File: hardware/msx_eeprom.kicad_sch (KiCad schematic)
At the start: 8 parts, among them J1 Conn_02x07_Odd_Even, P1 MSX_CONNECTOR, U1 AT28C256-15PU

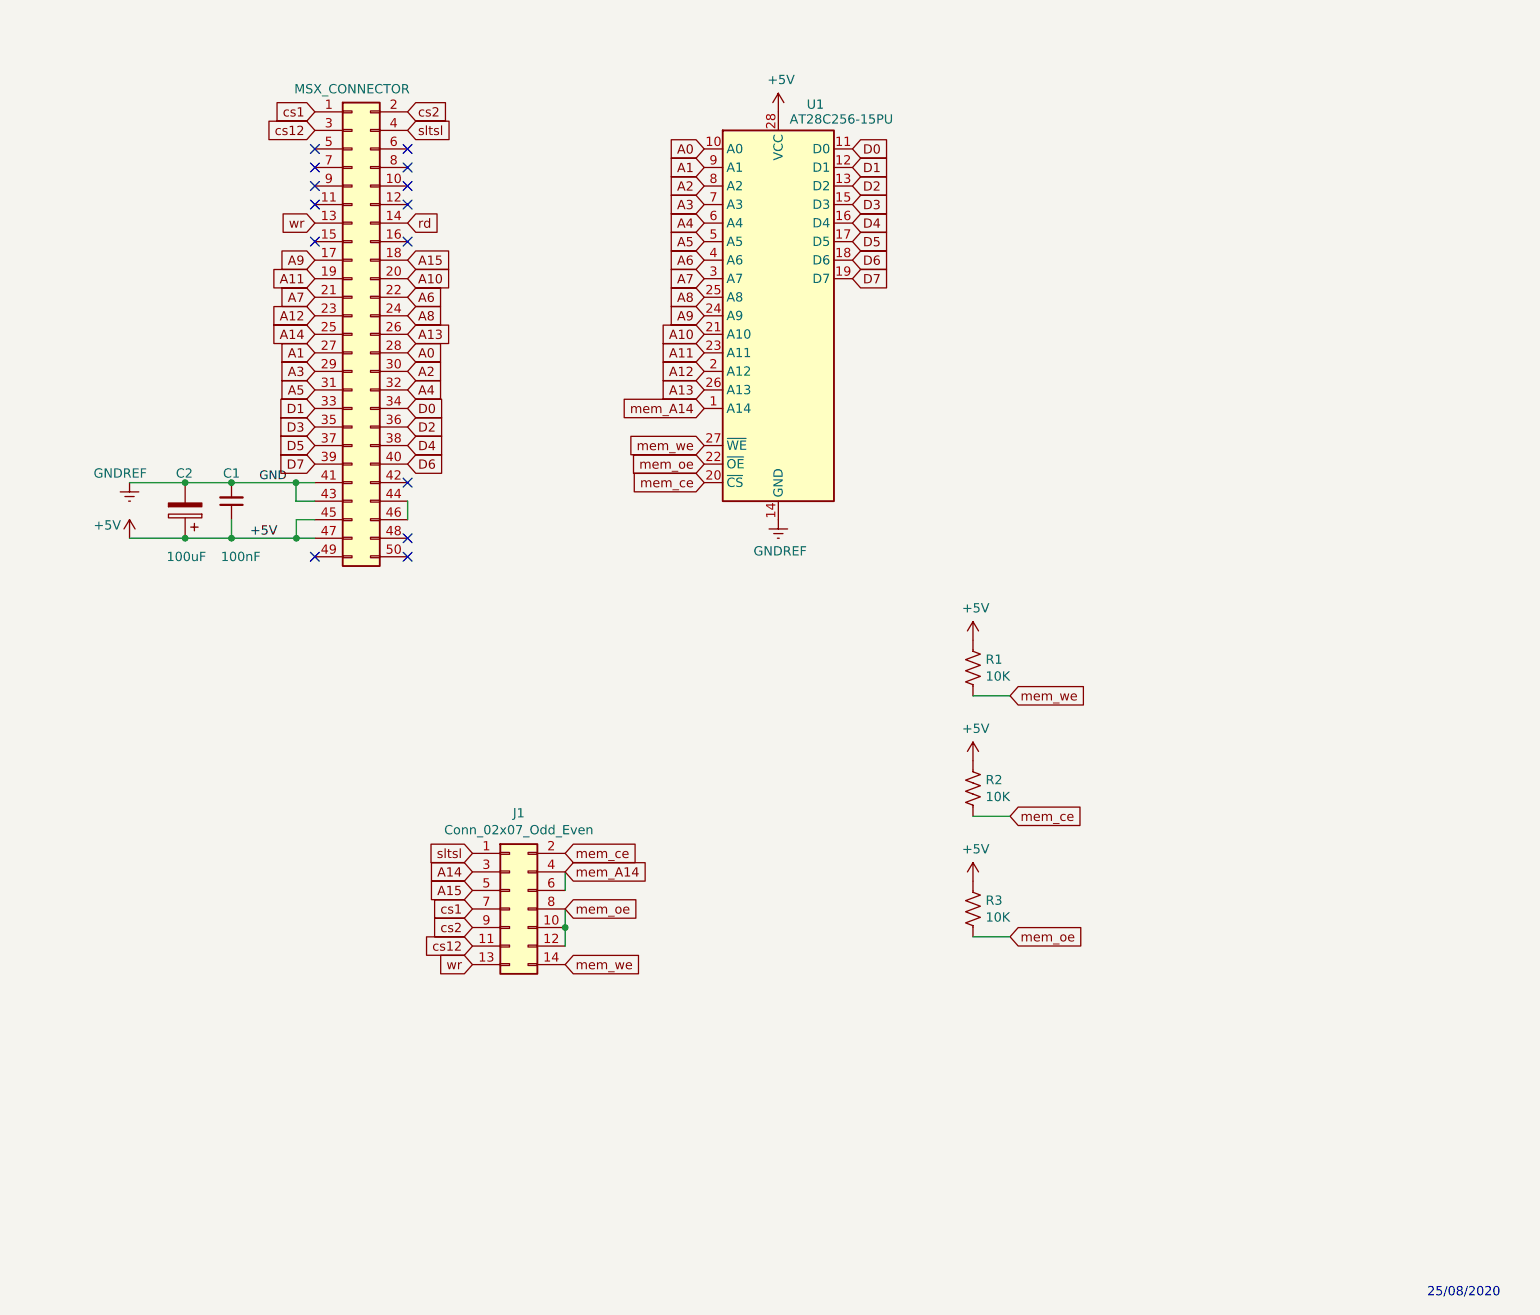
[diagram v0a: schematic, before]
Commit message: Rev 7
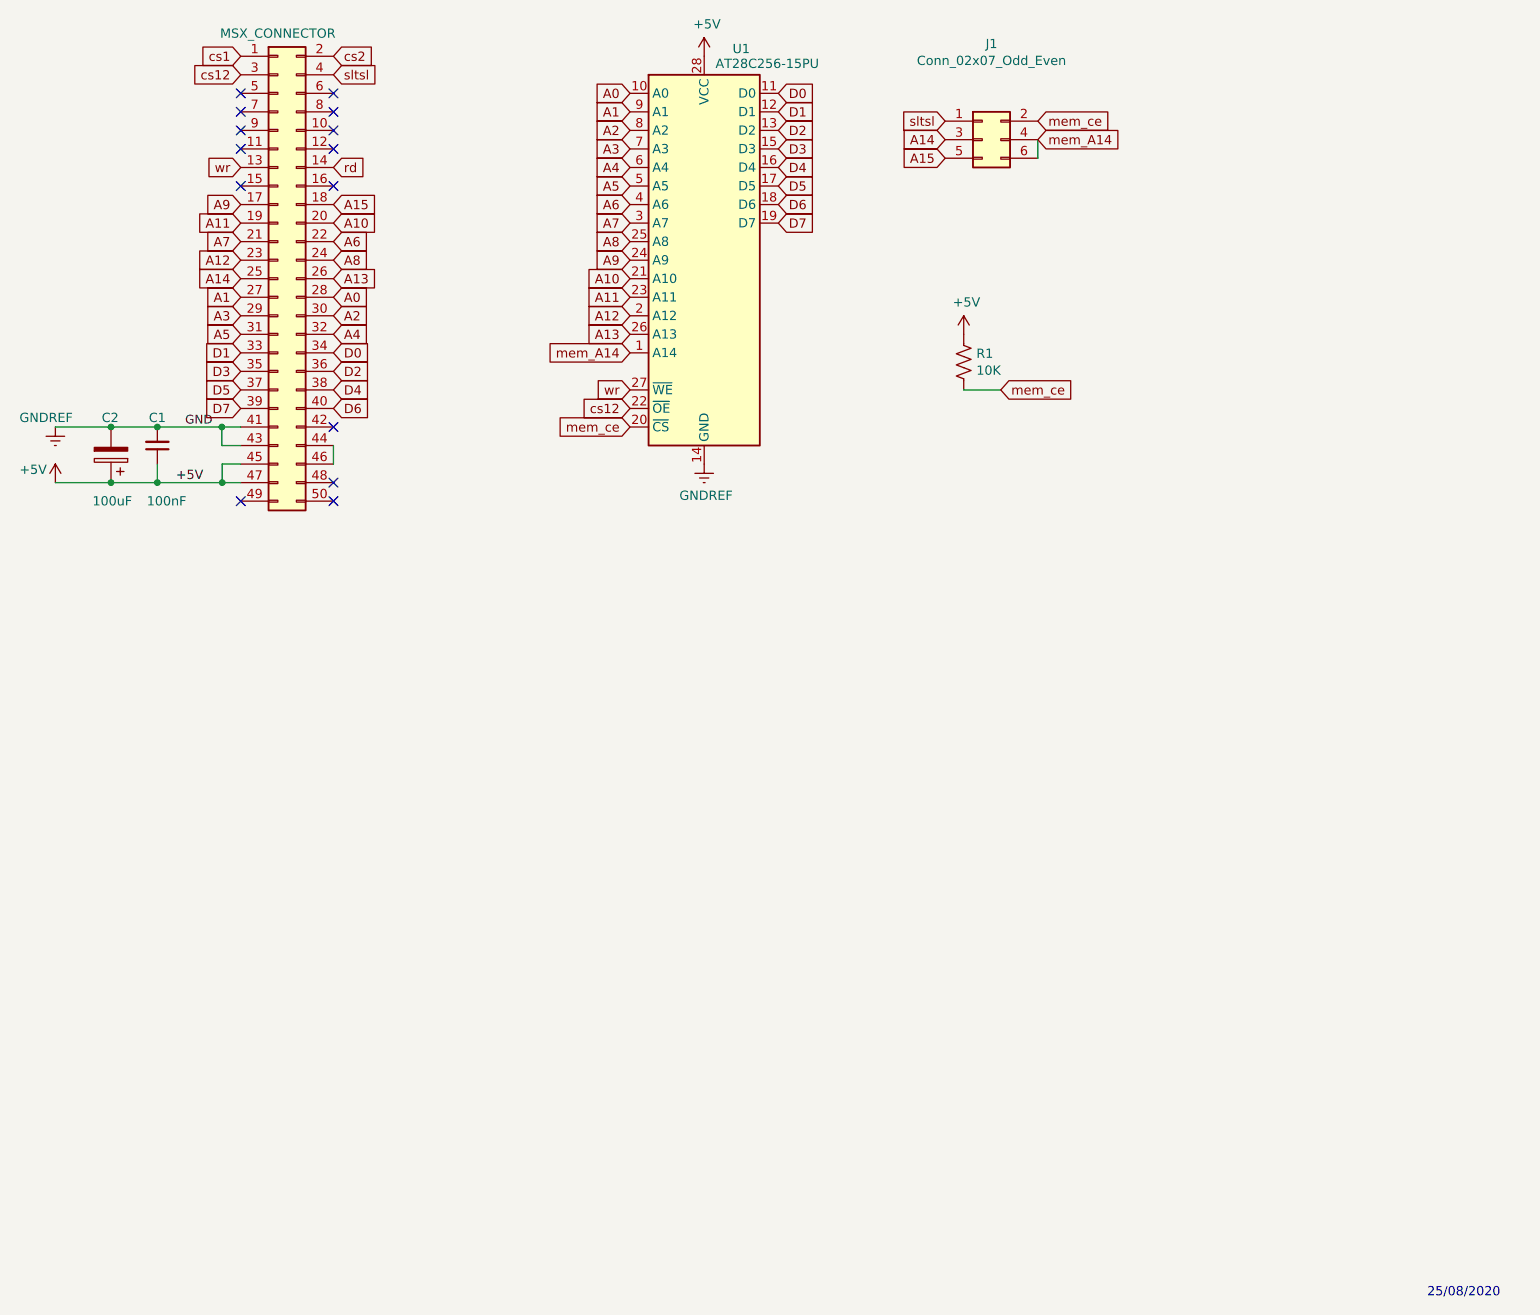
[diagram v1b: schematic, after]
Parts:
- removed R1, R3: 10K, Resistor_THT:R_Axial_DIN0207_L6.3mm_D2.5mm_P7.62mm_Horizontal, symbol Device:R_US
- J1: footprint Connector_PinHeader_2.54mm:PinHeader_2x07_P2.54mm_Horizontal -> Connector_PinHeader_2.54mm:PinHeader_2x03_P2.54mm_Horizontal; symbol Connector_Generic:Conn_02x07_Odd_Even -> Connector_Generic:Conn_02x03_Odd_Even
- P1: footprint MyFootprints:card_edge_connector -> Roni Footprints:MSX_CART_SW_Official
- renumbered R2 to R1
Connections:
- net cs1: no longer J1.7 (Pin_7)
- net cs12: now also U1.22 (~{OE}); no longer J1.11 (Pin_11)
- net cs2: no longer J1.9 (Pin_9)
- net wr: now also U1.27 (~{WE}); no longer J1.13 (Pin_13)
- removed net mem_oe: J1.10 (Pin_10), J1.12 (Pin_12), J1.8 (Pin_8), U1.22 (~{OE})
- removed net mem_we: J1.14 (Pin_14), U1.27 (~{WE})
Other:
- moved on the sheet: C1, C2, R1, U1

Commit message: Updated footprint to 2003 r1: pcb holes shiftted a little bit
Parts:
- P1: footprint Roni Footprints:MSX_CART_SW_Official -> Roni Footprints:MSX_CART_SW_Official_3Holes
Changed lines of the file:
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@@
   (title_block
     (title "MSX AT28C256 EEPROM Programable Cartridge")
-    (date "2023-02-28")
-    (rev "7")
+    (date "2023-03-17")
+    (rev "8")
     (company "RCC")
   )
@@
     )
     (property "Value" "MSX_CONNECTOR" (id 1) (at 50.8 21.0058 0))
-    (property "Footprint" "Roni Footprints:MSX_CART_SW_Official" (id 2) (at 50.8 54.61 0)
+    (property "Footprint" "Roni Footprints:MSX_CART_SW_Official_3Holes" (id 2) (at 50.8 54.61 0)
       (effects (font (size 1.27 1.27)) hide)
     )
@@
     )
     (path "/00000000-0000-0000-0000-00005edd120e"
-      (reference "P1") (unit 1) (value "MSX_CONNECTOR") (footprint "Roni Footprints:MSX_CART_SW_Official")
+      (reference "P1") (unit 1) (value "MSX_CONNECTOR") (footprint "Roni Footprints:MSX_CART_SW_Official_3Holes")
     )
     (path "/00000000-0000-0000-0000-00005f2edbce"
